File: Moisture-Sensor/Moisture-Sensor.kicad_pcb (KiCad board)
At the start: 2 copper layers, 20 x 100 mm, 20 parts, among them J1 Input, U1 LMV358, U2 NE555

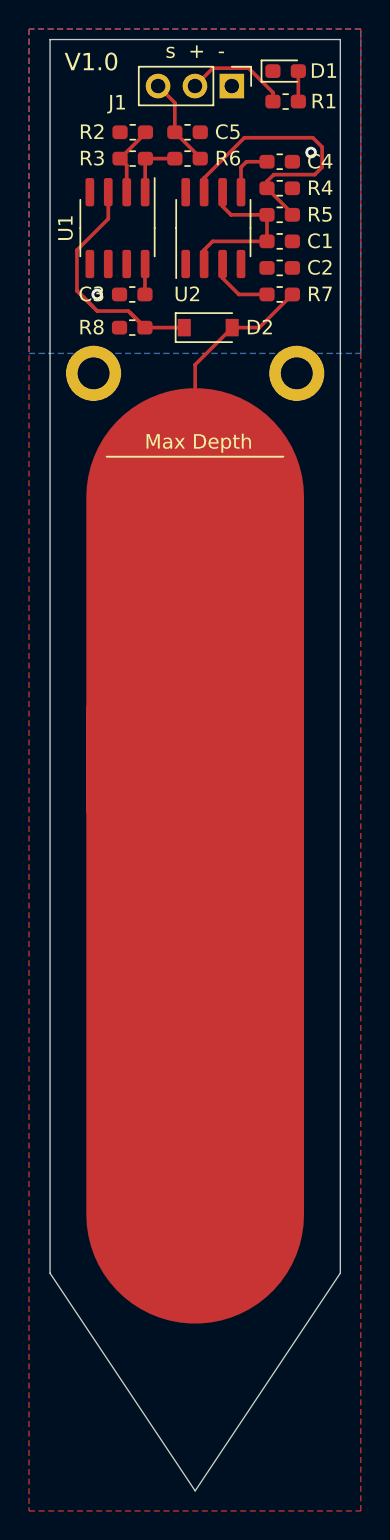
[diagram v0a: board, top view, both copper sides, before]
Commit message: Layout looks good and passed DRC
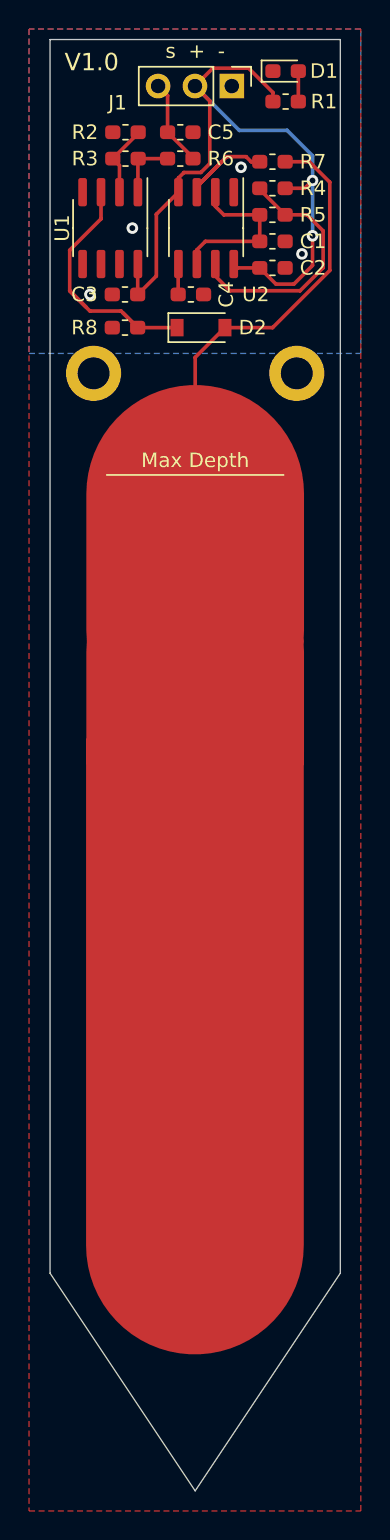
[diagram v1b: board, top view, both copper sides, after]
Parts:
- moved C4 11.0 mm to (109.7, 67.6)
- moved R7 9.16 mm to (115.3, 58.4)
- moved C1 0.50 mm to (115.3, 63.9)
- moved C2 0.50 mm to (115.3, 65.7)
- moved C3 0.50 mm to (105.2, 67.6)
- moved C5 0.50 mm to (109.0, 56.4)
- moved D2 0.50 mm to (110.4, 69.8)
- moved R2 0.50 mm to (105.2, 56.4)
- moved R3 0.50 mm to (105.2, 58.2)
- moved R4 0.50 mm to (115.3, 60.2)
- moved R5 0.50 mm to (115.3, 62.1)
- moved R6 0.50 mm to (109.0, 58.2)
- moved R8 0.50 mm to (105.2, 69.8)
- moved U1 0.50 mm to (104.1, 63.0)
- moved U2 0.50 mm to (110.8, 63.0), turned to 270 degrees
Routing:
- net +5V: track 9.30 -> 53.6 mm, vias 0 -> 2
- net Net-(D2-Pad2): track 72.3 -> 81.2 mm
- net Net-(R7-Pad1): track 4.50 -> 8.14 mm
- net Net-(R4-Pad2): track 19.1 -> 17.5 mm
- net Net-(C4-Pad2): track 3.67 -> 2.11 mm
- net GND: vias 2 -> 4
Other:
- net class Default: clearance 0.254 -> 0.2032
- rule trace_clearance: 0.254 -> 0.2032
